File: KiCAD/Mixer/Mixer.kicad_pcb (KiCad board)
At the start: 2 copper layers, 30 x 118.5 mm, 63 parts, among them J1 AudioJack2, J2 Conn_02x05_Odd_Even, J3 Conn_02x03_Odd_Even, J4 Conn_02x08_Odd_Even, J5 AudioJack2, Q1 MMBFJ111, Q2 MMBFJ111, Q3 MMBFJ111, Q4 MMBFJ111, SW1 SW_MEC_5G, SW2 SW_MEC_5G, U1 NE5532, U2 NE5532, U3 NE5532, U4 NE5532, U5 NE5532, U6 NE5532

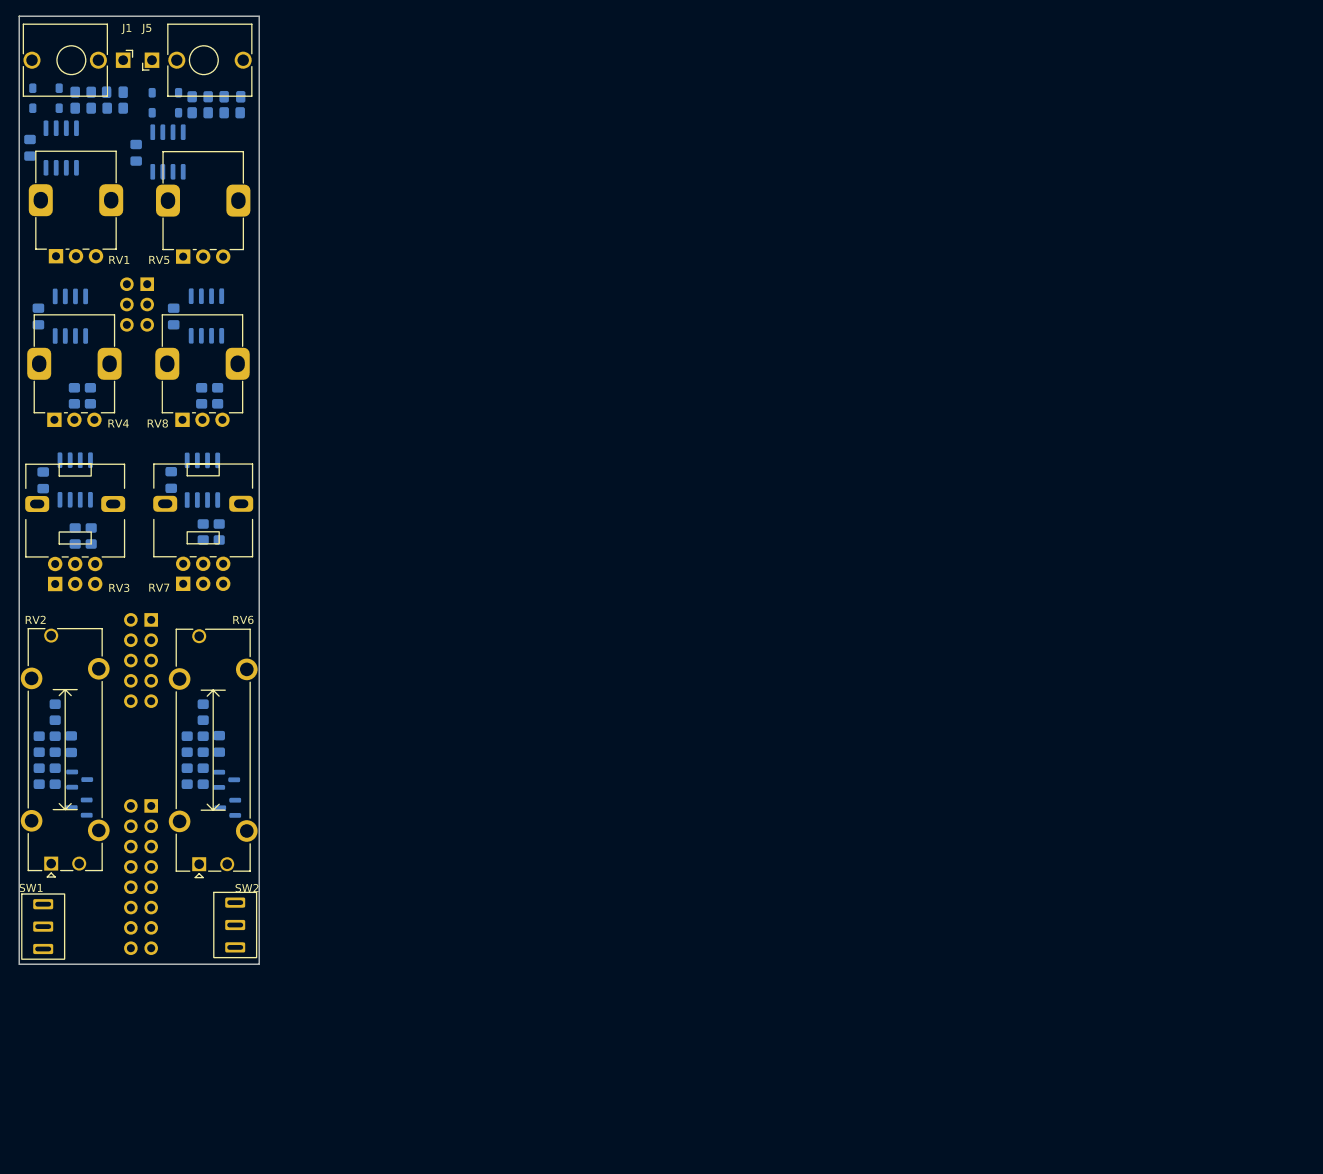
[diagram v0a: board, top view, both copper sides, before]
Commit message: überarbeitete Schaltung und PCB Desing...v1.0 FERTIG
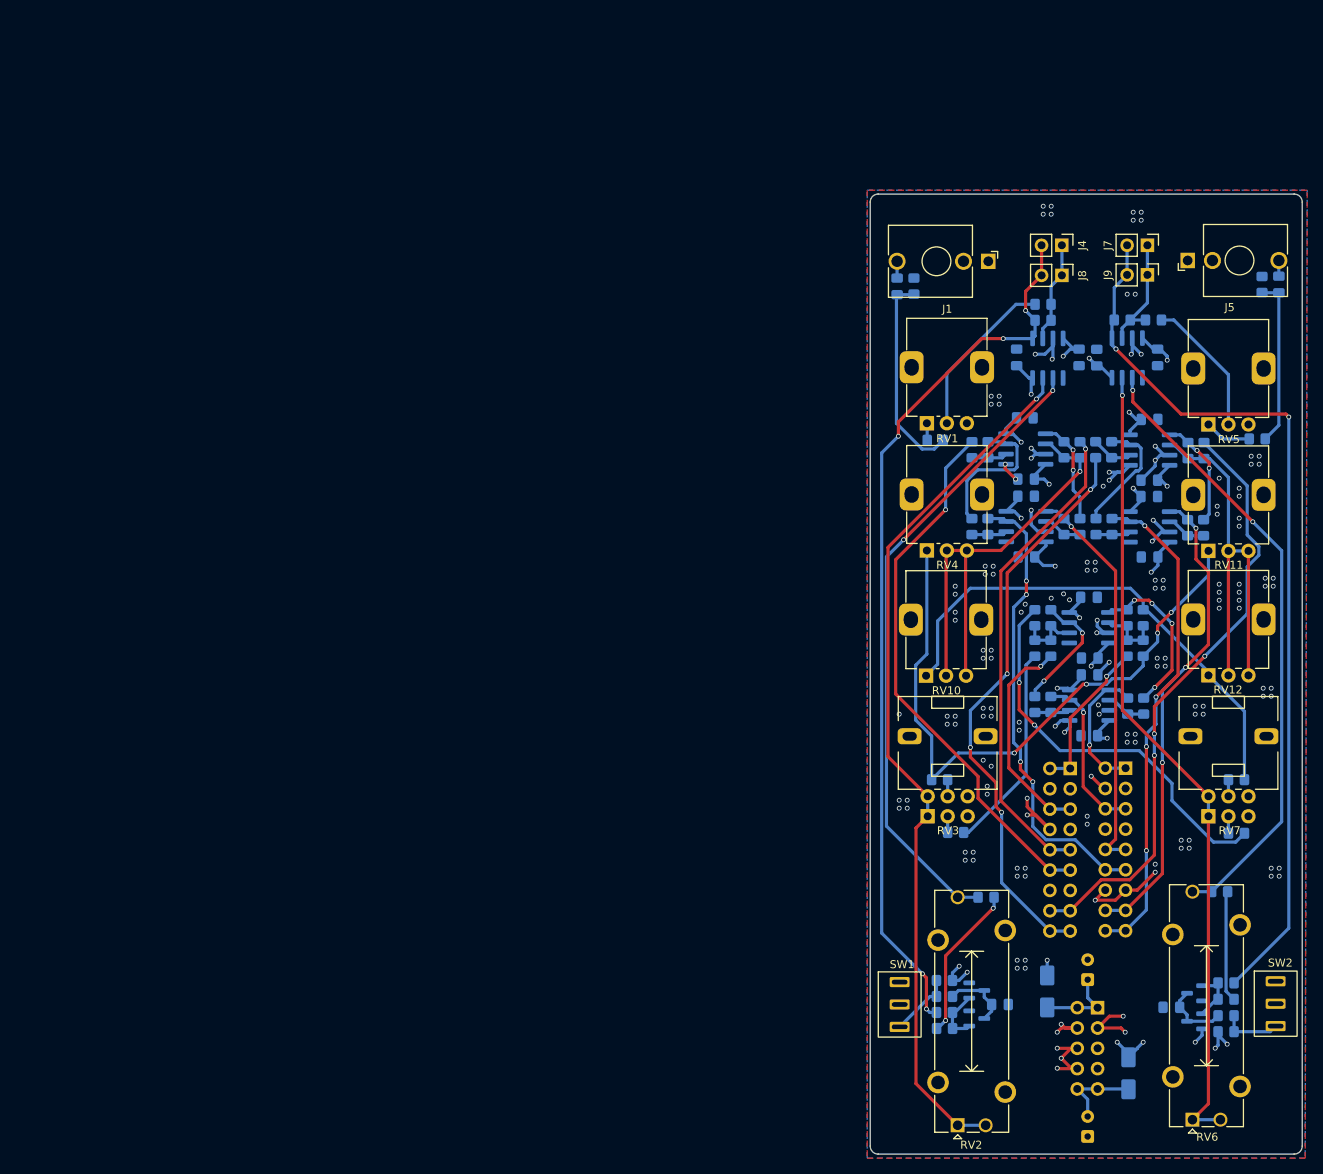
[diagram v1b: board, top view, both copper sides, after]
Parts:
- removed C2: 100n, Capacitor_SMD:C_0805_2012Metric_Pad1.18x1.45mm_HandSolder
- removed D1, D2, D5, D6: D, Diode_SMD:D_SOD-123
- removed J2: Conn_02x05_Odd_Even, Connector_PinHeader_2.54mm:PinHeader_2x05_P2.54mm_Vertical
- removed J3: Conn_02x03_Odd_Even, Connector_PinHeader_2.54mm:PinHeader_2x03_P2.54mm_Vertical
- removed RV8: 100, Potentiometer_THT:Potentiometer_Alps_RK09K_Single_Vertical
- added C11: 100n, Capacitor_SMD:C_0805_2012Metric_Pad1.18x1.45mm_HandSolder, B.Cu at (146.3, 55.4)
- added C12: 100n, Capacitor_SMD:C_0805_2012Metric_Pad1.18x1.45mm_HandSolder, B.Cu at (146.3, 65.0)
- added C13: 100n, Capacitor_SMD:C_0805_2012Metric_Pad1.18x1.45mm_HandSolder, B.Cu at (130.9, 62.9)
- added C14: 100n, Capacitor_SMD:C_0805_2012Metric_Pad1.18x1.45mm_HandSolder, B.Cu at (130.9, 72.6)
- added C15: 100n, Capacitor_SMD:C_0805_2012Metric_Pad1.18x1.45mm_HandSolder, B.Cu at (146.3, 63.0)
- added C16: 100n, Capacitor_SMD:C_0805_2012Metric_Pad1.18x1.45mm_HandSolder, B.Cu at (146.3, 72.6)
- added C17: 100u, Capacitor_THT:CP_Radial_D5.0mm_P2.50mm, B.Cu at (138.6, 125.4)
- added C33: 100n, Capacitor_SMD:C_0805_2012Metric_Pad1.18x1.45mm_HandSolder, B.Cu at (129.7, 47.6)
- added C34: 100n, Capacitor_SMD:C_0805_2012Metric_Pad1.18x1.45mm_HandSolder, B.Cu at (139.7, 47.7)
- added C35: 100n, Capacitor_SMD:C_0805_2012Metric_Pad1.18x1.45mm_HandSolder, B.Cu at (137.5, 47.6)
- added C37: 100n, Capacitor_SMD:C_0805_2012Metric_Pad1.18x1.45mm_HandSolder, B.Cu at (147.3, 47.6)
- added C40: 100n, Capacitor_SMD:C_0805_2012Metric_Pad1.18x1.45mm_HandSolder, B.Cu at (138.8, 85.2)
- added C41: 100n, Capacitor_SMD:C_0805_2012Metric_Pad1.18x1.45mm_HandSolder, B.Cu at (138.8, 94.9)
- added D3: 1N5711, Diode_SMD:D_SMA, B.Cu at (133.5, 126.9)
- added D4: 1N5711, Diode_SMD:D_SMA, B.Cu at (143.7, 137.1)
- added J10: Conn_02x09_Odd_Even, Connector_PinHeader_2.54mm:PinHeader_2x09_P2.54mm_Vertical, B.Cu at (143.3, 99.0)
- added J11: Conn_02x09_Odd_Even, Connector_PinHeader_2.54mm:PinHeader_2x09_P2.54mm_Vertical, B.Cu at (136.4, 99.0)
- added J6: Conn_02x05_Odd_Even, Connector_PinHeader_2.54mm:PinHeader_2x05_P2.54mm_Vertical, B.Cu at (139.8, 128.9)
- added J7: Conn_01x02_Socket, Connector_PinHeader_2.54mm:PinHeader_1x02_P2.54mm_Vertical, F.Cu at (146.0, 33.6)
- added J8: Conn_01x02_Socket, Connector_PinHeader_2.54mm:PinHeader_1x02_P2.54mm_Vertical, F.Cu at (135.3, 37.4)
- added J9: Conn_01x02_Socket, Connector_PinHeader_2.54mm:PinHeader_1x02_P2.54mm_Vertical, F.Cu at (146.0, 37.3)
- added R25: 1k, Resistor_SMD:R_0805_2012Metric_Pad1.20x1.40mm_HandSolder, B.Cu at (151.1, 59.3)
- added R26: 1k, Resistor_SMD:R_0805_2012Metric_Pad1.20x1.40mm_HandSolder, B.Cu at (141.6, 59.2)
- added R29: 1k, Resistor_SMD:R_0805_2012Metric_Pad1.20x1.40mm_HandSolder, B.Cu at (143.5, 80.2)
- added R30: 1k, Resistor_SMD:R_0805_2012Metric_Pad1.20x1.40mm_HandSolder, B.Cu at (134.0, 80.2)
- added R31: 1k, Resistor_SMD:R_0805_2012Metric_Pad1.20x1.40mm_HandSolder, B.Cu at (132.0, 84.0)
- added R32: 1k, Resistor_SMD:R_0805_2012Metric_Pad1.20x1.40mm_HandSolder, B.Cu at (132.0, 80.2)
- added R33: 1k, Resistor_SMD:R_0805_2012Metric_Pad1.20x1.40mm_HandSolder, B.Cu at (145.5, 80.2)
- added R34: 1k, Resistor_SMD:R_0805_2012Metric_Pad1.20x1.40mm_HandSolder, B.Cu at (145.5, 84.0)
- added R35: 1k, Resistor_SMD:R_0805_2012Metric_Pad1.20x1.40mm_HandSolder, B.Cu at (143.5, 84.0)
- added R36: 1k, Resistor_SMD:R_0805_2012Metric_Pad1.20x1.40mm_HandSolder, B.Cu at (134.0, 84.0)
- added R37: 1k, Resistor_SMD:R_0805_2012Metric_Pad1.20x1.40mm_HandSolder, B.Cu at (143.6, 91.2)
- added R38: 1k, Resistor_SMD:R_0805_2012Metric_Pad1.20x1.40mm_HandSolder, B.Cu at (134.0, 91.0)
- added R39: 1k, Resistor_SMD:R_0805_2012Metric_Pad1.20x1.40mm_HandSolder, B.Cu at (124.1, 59.2)
- added R40: 1k, Resistor_SMD:R_0805_2012Metric_Pad1.20x1.40mm_HandSolder, B.Cu at (139.6, 59.2)
- added R41: 1k, Resistor_SMD:R_0805_2012Metric_Pad1.20x1.40mm_HandSolder, B.Cu at (132.0, 91.0)
- added R42: 1k, Resistor_SMD:R_0805_2012Metric_Pad1.20x1.40mm_HandSolder, B.Cu at (145.6, 91.2)
- added R43: 1k, Resistor_SMD:R_0805_2012Metric_Pad1.20x1.40mm_HandSolder, B.Cu at (137.6, 59.2)
- added R44: 1k, Resistor_SMD:R_0805_2012Metric_Pad1.20x1.40mm_HandSolder, B.Cu at (153.1, 59.3)
- added R45: 1k, Resistor_SMD:R_0805_2012Metric_Pad1.20x1.40mm_HandSolder, B.Cu at (139.6, 68.8)
- added R46: 1k, Resistor_SMD:R_0805_2012Metric_Pad1.20x1.40mm_HandSolder, B.Cu at (153.1, 68.9)
- added R47: 1k, Resistor_SMD:R_0805_2012Metric_Pad1.20x1.40mm_HandSolder, B.Cu at (151.1, 68.9)
- added R48: 1k, Resistor_SMD:R_0805_2012Metric_Pad1.20x1.40mm_HandSolder, B.Cu at (141.6, 68.8)
- added R49: 1k, Resistor_SMD:R_0805_2012Metric_Pad1.20x1.40mm_HandSolder, B.Cu at (124.1, 68.8)
- added R50: 1k, Resistor_SMD:R_0805_2012Metric_Pad1.20x1.40mm_HandSolder, B.Cu at (137.6, 68.8)
- added R51: 1k, Resistor_SMD:R_0805_2012Metric_Pad1.20x1.40mm_HandSolder, B.Cu at (135.6, 68.8)
- added R52: 1k, Resistor_SMD:R_0805_2012Metric_Pad1.20x1.40mm_HandSolder, B.Cu at (126.1, 68.8)
- added RV10: 1k, Potentiometer_THT:Potentiometer_Alps_RK09K_Single_Vertical, F.Cu at (118.4, 87.4)
- added RV11: 1k, Potentiometer_THT:Potentiometer_Alps_RK09K_Single_Vertical, F.Cu at (153.7, 71.8)
- added RV12: 1k, Potentiometer_THT:Potentiometer_Alps_RK09K_Single_Vertical, F.Cu at (153.7, 87.4)
- added U7: NE5532, Package_SO:SOIC-8_3.9x4.9mm_P1.27mm, B.Cu at (146.3, 59.2)
- added U8: NE5532, Package_SO:SOIC-8_3.9x4.9mm_P1.27mm, B.Cu at (146.3, 68.8)
- C1, C3: value 470u -> 4,7
- C4, C6: value 100n -> 220n
- C5: value 100n -> 100u; footprint Capacitor_SMD:C_0805_2012Metric_Pad1.18x1.45mm_HandSolder -> Capacitor_THT:CP_Radial_D5.0mm_P2.50mm
- J4: value Conn_02x08_Odd_Even -> Conn_01x02_Socket; footprint Connector_PinHeader_2.54mm:PinHeader_2x08_P2.54mm_Vertical -> Connector_PinHeader_2.54mm:PinHeader_1x02_P2.54mm_Vertical; moved to F.Cu
- R1, R13, R15, R3: value R -> 10k
- R11, R12: value 100 -> R
- R14, R2: value R -> 1k
- R23, R24, RV4: value 100 -> 1k
- moved C5 171.1 mm to (138.6, 145.0), turned to 90 degrees
- moved R12 147.1 mm to (160.4, 38.5), turned to -90 degrees
- moved R13 134.5 mm to (159.8, 57.8)
- moved R18 134.2 mm to (155.9, 129.9), turned to 180 degrees
- moved R16 133.7 mm to (155.9, 131.9), turned to 0 degrees
- moved J4 133.7 mm to (135.3, 33.6), turned to -90 degrees
- moved C3 132.9 mm to (162.5, 38.5), turned to -90 degrees
- moved R21 132.8 mm to (157.2, 100.4), turned to 0 degrees
- moved R22 132.6 mm to (157.2, 107.1), turned to 0 degrees
- moved J5 131.9 mm to (151.1, 35.5)
- moved R19 131.8 mm to (155.9, 127.9), turned to 0 degrees
- moved C9 131.5 mm to (138.7, 77.6), turned to 180 degrees
- moved RV7 131.4 mm to (153.7, 105.0)
- moved R17 130.4 mm to (155.9, 125.8), turned to 180 degrees
- moved SW2 130.4 mm to (159.4, 124.4)
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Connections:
- C10 pad 2: +12V -> /Channel/+12V
- C5 pad 2: +12V -> Net-(D4-K)
- C7 pad 2: +12V -> /Channel/+12V
- C8 pad 2: +12V -> /Channel/+12V
- C9 pad 2: +12V -> /Channel/+12V
- J4 pad 1: -12V -> Net-(J4-Pin_1)
- J4 pad 2: -12V -> /Channel/Gain/gain_out
- R1 pad 1: Net-(D1-K) -> Net-(J4-Pin_1)
- R10 pad 2: /Channel/Main Mix/main_inR -> /Channel/Ch1_outR
- R11 pad 1: /Channel/Main Mix/main_inL -> GND
- R11 pad 2: Net-(U3A-+) -> /Channel/Gain/gain_in
- R12 pad 1: /Channel/Main Mix/main_inR -> GND
- R12 pad 2: Net-(U3B-+) -> /Channel/Gain1/gain_in
- R2 pad 2: Net-(D1-K) -> Net-(J4-Pin_1)
- R21 pad 2: /Channel/Main Mix1/main_inL -> /Channel/Ch2_outL
- R22 pad 2: /Channel/Main Mix1/main_inR -> /Channel/Ch2_outR
- R23 pad 1: /Channel/Main Mix1/main_inL -> Net-(U3B--)
- R23 pad 2: Net-(U5A-+) -> Net-(R23-Pad2)
- R24 pad 1: /Channel/Main Mix1/main_inR -> Net-(U3A--)
- R24 pad 2: Net-(U5B-+) -> Net-(R24-Pad2)
- R9 pad 2: /Channel/Main Mix/main_inL -> /Channel/Ch1_outL
- RV4 pad 1: Net-(U3A--) -> /Channel/Ch1_outL
- RV4 pad 2: /Channel/ch1send_L -> Net-(U3A--)
- RV4 pad 3: /Channel/ch1send_L -> Net-(U3A--)
- SW1 pad 1: -12V -> /Channel/-12V
- SW1 pad 2: -12V -> /Channel/-12V
- SW2 pad 1: -12V -> /Channel/-12V
- SW2 pad 2: -12V -> /Channel/-12V
- U1 pad 2: Net-(D1-K) -> Net-(J4-Pin_1)
- U1 pad 4: -12V -> /Channel/-12V
- U1 pad 8: +12V -> /Channel/+12V
- U2 pad 4: -12V -> /Channel/-12V
- U2 pad 8: +12V -> /Channel/+12V
- U3 pad 1: /Channel/ch1send_L -> Net-(R24-Pad2)
- U3 pad 3: Net-(U3A-+) -> GND
- U3 pad 4: -12V -> /Channel/-12V
- U3 pad 5: Net-(U3B-+) -> GND
- U3 pad 7: /Channel/ch1send_R -> Net-(R23-Pad2)
- U3 pad 8: +12V -> /Channel/+12V
- U4 pad 1: /Channel/ch1out_L -> Net-(R29-Pad2)
- U4 pad 2: /Channel/ch1out_L -> Net-(U4A--)
- U4 pad 3: /Channel/Main Mix/main_inL -> GND
- U4 pad 4: -12V -> /Channel/-12V
- U4 pad 5: /Channel/Main Mix/main_inR -> GND
- U4 pad 6: /Channel/ch1out_R -> Net-(U4B--)
- U4 pad 7: /Channel/ch1out_R -> Net-(R30-Pad2)
- U4 pad 8: +12V -> /Channel/+12V
- U5 pad 1: /Channel/ch1send_L -> /Channel/main_mixL
- U5 pad 3: Net-(U5A-+) -> GND
- U5 pad 4: -12V -> /Channel/-12V
- U5 pad 5: Net-(U5B-+) -> GND
- U5 pad 7: /Channel/ch1send_R -> /Channel/main_mixR
- U5 pad 8: +12V -> /Channel/+12V
- U6 pad 1: /Channel/ch1out_L -> /Channel/send_out1L
- U6 pad 2: /Channel/ch1out_L -> Net-(U6A--)
- U6 pad 3: /Channel/Main Mix1/main_inL -> GND
- U6 pad 4: -12V -> /Channel/-12V
- U6 pad 5: /Channel/Main Mix1/main_inR -> GND
- U6 pad 6: /Channel/ch1out_R -> Net-(U6B--)
- U6 pad 7: /Channel/ch1out_R -> /Channel/send_out1R
- U6 pad 8: +12V -> /Channel/+12V
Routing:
- net /Channel/-12V: track 0.00 -> 224.4 mm, vias 0 -> 10
- net /Channel/+12V: track 0.00 -> 143.8 mm, vias 0 -> 9
- net /Channel/Gain1/gain_out: track 0.00 -> 112.7 mm, vias 0 -> 2
- net /Channel/Gain/gain_out: track 0.00 -> 112.2 mm, vias 0 -> 5
- net /Channel/Fader/fader_out: track 0.00 -> 109.7 mm, vias 0 -> 1
- net GND: track 0.00 -> 104.5 mm, vias 0 -> 160
- net /Channel/Fader1/fader_out: track 0.00 -> 101.5 mm, vias 0 -> 1
- net /Channel/Ch1_outL: track 0.00 -> 80.1 mm, vias 0 -> 4
- net Net-(U1B--): track 0.00 -> 79.8 mm, vias 0 -> 2
- net Net-(U2B--): track 0.00 -> 78.0 mm, vias 0 -> 2
- net /Channel/pre_send2L: track 0.00 -> 75.8 mm, vias 0 -> 3
- net /Channel/pre_send2R: track 0.00 -> 72.3 mm, vias 0 -> 4
- net /Channel/pre_send1R: track 0.00 -> 68.0 mm, vias 0 -> 1
- net /Channel/Ch2_outL: track 0.00 -> 64.0 mm
- net /Channel/send_out2R: track 0.00 -> 62.1 mm, vias 0 -> 4
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- added copper zone on B.Cu, net GND
- added copper zone on F.Cu, net GND
- added copper zone on In1.Cu, net GND
- added copper zone on In2.Cu, net GND
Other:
- board size 30 x 118.5 mm -> 54 x 120 mm
- copper layers 2 -> 4
